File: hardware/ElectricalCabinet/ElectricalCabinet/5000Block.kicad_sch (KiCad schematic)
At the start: 0 parts

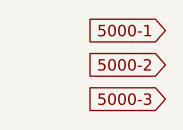
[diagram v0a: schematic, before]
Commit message: More updates
Added drawing sheets, wire label scheme, signal list, and traffic light label image to docs folder
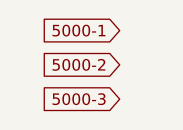
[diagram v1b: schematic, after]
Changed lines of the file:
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@@
 	(global_label "5000-1"
 		(shape input)
-		(at 60.96 6.35 180)
+		(at 55.88 6.35 180)
 		(effects
 			(font
@@
 		)
 		(property "Intersheetrefs" "109"
-			(at 50.3549 6.35 0)
+			(at 45.2749 6.35 0)
 			(hide yes)
 			(show_name no)
@@
 		)
 		(property "Ref" "Ref 109"
-			(at 50.8 6.35 0)
+			(at 45.72 6.35 0)
 			(show_name no)
 			(do_not_autoplace no)
@@
 	(global_label "5000-3"
 		(shape input)
-		(at 60.96 13.97 180)
+		(at 55.88 13.97 180)
 		(effects
 			(font
@@
 		)
 		(property "Intersheetrefs" "333"
-			(at 50.3549 13.97 0)
+			(at 45.2749 13.97 0)
 			(hide yes)
 			(show_name no)
@@
 		)
 		(property "Ref" "Ref 333"
-			(at 42.926 13.97 0)
+			(at 37.846 13.97 0)
 			(show_name no)
 			(do_not_autoplace no)
@@
 	(global_label "5000-2"
 		(shape input)
-		(at 60.96 10.16 180)
+		(at 55.88 10.16 180)
 		(effects
 			(font
@@
 		)
 		(property "Intersheetrefs" "212"
-			(at 50.3549 10.16 0)
+			(at 45.2749 10.16 0)
 			(hide yes)
 			(show_name no)
@@
 		)
 		(property "Ref" "Ref 212"
-			(at 42.926 10.16 0)
+			(at 37.846 10.16 0)
 			(show_name no)
 			(do_not_autoplace no)
